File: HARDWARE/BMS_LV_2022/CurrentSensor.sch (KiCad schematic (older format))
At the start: 3 parts, among them U5 ACHS-7123

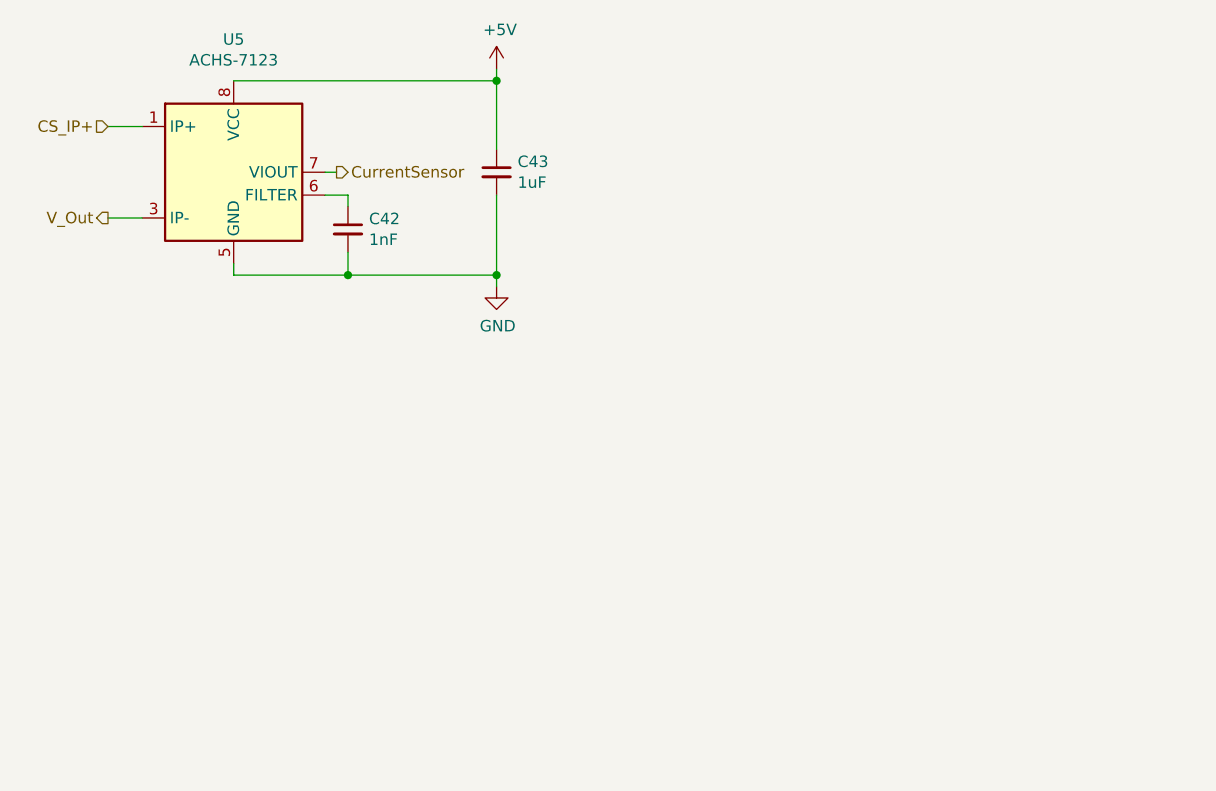
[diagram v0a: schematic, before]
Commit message: Most of the footprints added
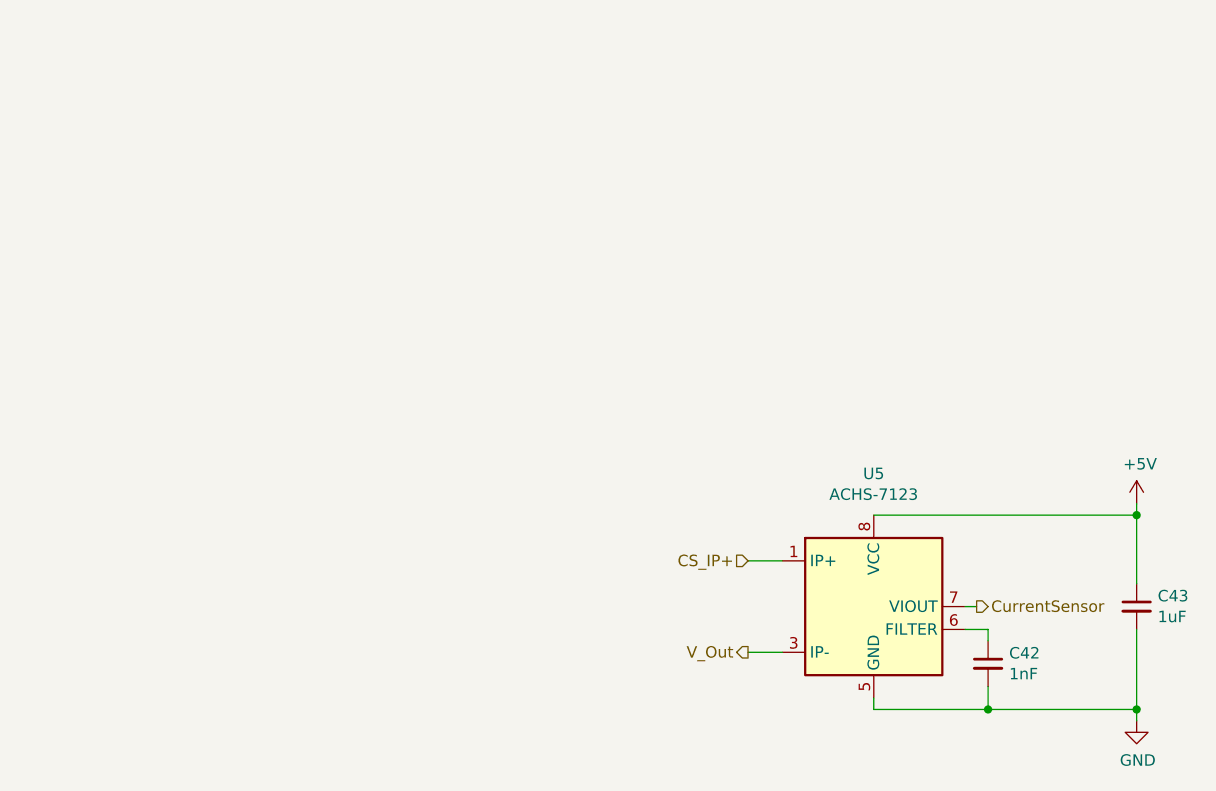
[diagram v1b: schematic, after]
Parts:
- C42, C43: footprint (none) -> Capacitor_SMD:C_0603_1608Metric
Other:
- moved on the sheet: C42, C43, U5
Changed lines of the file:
@@
 EELAYER 30 0
 EELAYER END
-$Descr User 5906 4725
+$Descr A4 11693 8268
 encoding utf-8
 Sheet 13 13
@@
 L Sensor_Current:ACS712xLCTR-30A U?
 U 1 1 62C41044
-P 2600 1800
+P 5400 3700
 AR Path="/62C41044" Ref="U?"  Part="1"
 AR Path="/62C2DD72/62C41044" Ref="U5"  Part="1"
-F 0 "U5" H 2600 2381 50  0000 C CNN
-F 1 "ACHS-7123" H 2600 2290 50  0000 C CNN
-F 2 "Package_SO:SOIC-8_3.9x4.9mm_P1.27mm" H 2700 1450 50  0001 L CIN
-F 3 "https://download.kamami.pl/p586603-ACHS-712x-DS101_2018-02-28.pdf" H 2600 1800 50  0001 C CNN
-	1    2600 1800
+F 0 "U5" H 5400 4281 50  0000 C CNN
+F 1 "ACHS-7123" H 5400 4190 50  0000 C CNN
+F 2 "Package_SO:SOIC-8_3.9x4.9mm_P1.27mm" H 5500 3350 50  0001 L CIN
+F 3 "https://download.kamami.pl/p586603-ACHS-712x-DS101_2018-02-28.pdf" H 5400 3700 50  0001 C CNN
+	1    5400 3700
 	1    0    0    -1
 $EndComp
 Wire Wire Line
-	2200 1600 2050 1600
+	5000 3500 4850 3500
 Wire Wire Line
-	2200 2000 2050 2000
+	5000 3900 4850 3900
 Wire Wire Line
-	2600 2200 2600 2250
+	5400 4100 5400 4150
 $Comp
 L Device:C_Small C?
 U 1 1 62C4104D
-P 3100 2050
+P 5900 3950
 AR Path="/62C4104D" Ref="C?"  Part="1"
 AR Path="/62C2DD72/62C4104D" Ref="C42"  Part="1"
-F 0 "C42" H 3192 2096 50  0000 L CNN
-F 1 "1nF" H 3192 2005 50  0000 L CNN
-F 2 "" H 3100 2050 50  0001 C CNN
-F 3 "~" H 3100 2050 50  0001 C CNN
-	1    3100 2050
+F 0 "C42" H 5992 3996 50  0000 L CNN
+F 1 "1nF" H 5992 3905 50  0000 L CNN
+F 2 "Capacitor_SMD:C_0603_1608Metric" H 5900 3950 50  0001 C CNN
+F 3 "~" H 5900 3950 50  0001 C CNN
+	1    5900 3950
 	1    0    0    -1
 $EndComp
 Wire Wire Line
-	3000 1900 3100 1900
+	5800 3800 5900 3800
 Wire Wire Line
-	3100 1900 3100 1950
+	5900 3800 5900 3850
 Wire Wire Line
-	3100 2150 3100 2250
+	5900 4050 5900 4150
 Wire Wire Line
-	2600 2250 3100 2250
+	5400 4150 5900 4150
 Wire Wire Line
-	3000 1800 3050 1800
+	5800 3700 5850 3700
 $Comp
 L Device:C_Small C?
 U 1 1 62C4105A
-P 3750 1800
+P 6550 3700
 AR Path="/62C4105A" Ref="C?"  Part="1"
 AR Path="/62C2DD72/62C4105A" Ref="C43"  Part="1"
-F 0 "C43" H 3842 1846 50  0000 L CNN
-F 1 "1uF" H 3842 1755 50  0000 L CNN
-F 2 "" H 3750 1800 50  0001 C CNN
-F 3 "~" H 3750 1800 50  0001 C CNN
-	1    3750 1800
+F 0 "C43" H 6642 3746 50  0000 L CNN
+F 1 "1uF" H 6642 3655 50  0000 L CNN
+F 2 "Capacitor_SMD:C_0603_1608Metric" H 6550 3700 50  0001 C CNN
+F 3 "~" H 6550 3700 50  0001 C CNN
+	1    6550 3700
 	1    0    0    -1
 $EndComp
 Wire Wire Line
-	3750 2250 3750 1900
+	6550 4150 6550 3800
 Wire Wire Line
-	3750 1700 3750 1400
+	6550 3600 6550 3300
 $Comp
 L power:GND #PWR?
 U 1 1 62C41064
-P 3750 2300
+P 6550 4200
 AR Path="/62C41064" Ref="#PWR?"  Part="1"
 AR Path="/62C2DD72/62C41064" Ref="#PWR050"  Part="1"
-F 0 "#PWR050" H 3750 2050 50  0001 C CNN
-F 1 "GND" H 3755 2127 50  0000 C CNN
-F 2 "" H 3750 2300 50  0001 C CNN
-F 3 "" H 3750 2300 50  0001 C CNN
-	1    3750 2300
+F 0 "#PWR050" H 6550 3950 50  0001 C CNN
+F 1 "GND" H 6555 4027 50  0000 C CNN
+F 2 "" H 6550 4200 50  0001 C CNN
+F 3 "" H 6550 4200 50  0001 C CNN
+	1    6550 4200
 	1    0    0    -1
 $EndComp
 Wire Wire Line
-	3750 2250 3750 2300
-Connection ~ 3750 2250
+	6550 4150 6550 4200
+Connection ~ 6550 4150
 $Comp
 L power:+5V #PWR?
 U 1 1 62C4106C
-P 3750 1350
+P 6550 3250
 AR Path="/62C4106C" Ref="#PWR?"  Part="1"
 AR Path="/62C2DD72/62C4106C" Ref="#PWR049"  Part="1"
-F 0 "#PWR049" H 3750 1200 50  0001 C CNN
-F 1 "+5V" H 3765 1523 50  0000 C CNN
-F 2 "" H 3750 1350 50  0001 C CNN
-F 3 "" H 3750 1350 50  0001 C CNN
-	1    3750 1350
+F 0 "#PWR049" H 6550 3100 50  0001 C CNN
+F 1 "+5V" H 6565 3423 50  0000 C CNN
+F 2 "" H 6550 3250 50  0001 C CNN
+F 3 "" H 6550 3250 50  0001 C CNN
+	1    6550 3250
 	1    0    0    -1
 $EndComp
 Wire Wire Line
-	3750 1350 3750 1400
-Connection ~ 3750 1400
-Text HLabel 2050 1600 0    50   Input ~ 0
+	6550 3250 6550 3300
+Connection ~ 6550 3300
+Text HLabel 4850 3500 0    50   Input ~ 0
 CS_IP+
-Text HLabel 2050 2000 0    50   Output ~ 0
+Text HLabel 4850 3900 0    50   Output ~ 0
 V_Out
-Text HLabel 3050 1800 2    50   Output ~ 0
+Text HLabel 5850 3700 2    50   Output ~ 0
 CurrentSensor
 Wire Wire Line
-	3100 2250 3750 2250
-Connection ~ 3100 2250
+	5900 4150 6550 4150
+Connection ~ 5900 4150
 Wire Wire Line
-	2600 1400 3750 1400
+	5400 3300 6550 3300
 $EndSCHEMATC
